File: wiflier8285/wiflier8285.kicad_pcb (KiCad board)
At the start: 2 copper layers, 37.8 x 21.5 mm, 46 parts, among them CN1 1u, CN2 1u, M0 M, M1 M, M2 M, M3 M, P1 USBMicroB-10118194-0001LF, P2 CONN_01X02, P3 I2C, P4 TXRX, P5 TXRX, P6 IVP, P7 M, P8 M, P9 SYSRESET, Q0 NFET, Q1 NFET, Q2 NFET, Q3 NFET, U1 BMP280, U2 ESP8285, U3 LSM9DS1, U4 MCP1824v3.3, U5 MCP1824v3.3, U6 MCP1824v2.5, U7 STBC08, X1 XTAL4P

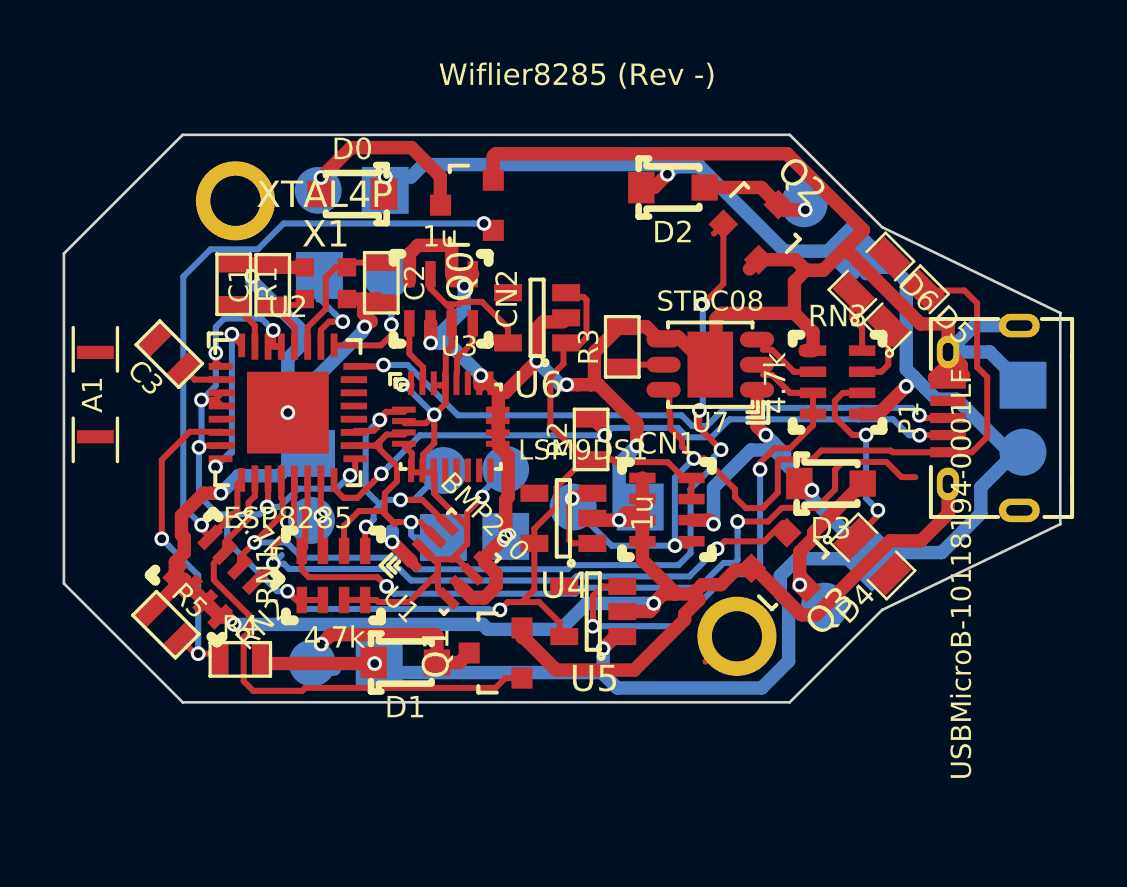
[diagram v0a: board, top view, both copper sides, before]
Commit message: Update!
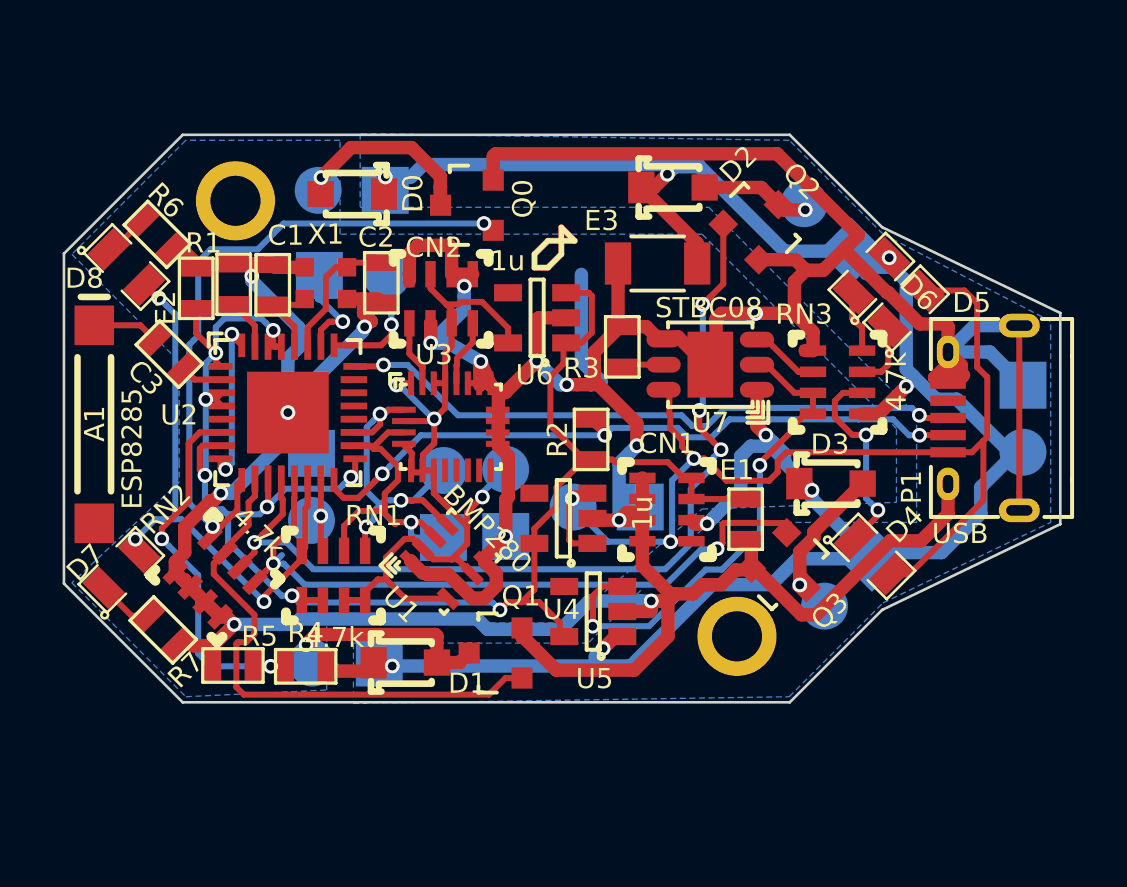
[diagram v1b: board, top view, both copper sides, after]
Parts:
- added D7: BLU, SM0805, F.Cu at (47.6, 65.7)
- added D8: BLU, SM0805, F.Cu at (47.8, 54.2)
- added E1: 10u, SM0603, F.Cu at (71.3, 63.7)
- added E2: 10u, SM0603, F.Cu at (50.5, 55.0)
- added E3: 100u, C_1206, F.Cu at (67.9, 54.1)
- added R6: 1.5k, SM0603, F.Cu at (49.0, 52.9)
- added R7: 1.5k, SM0603, F.Cu at (49.2, 67.9)
- A1: footprint ANT1206 -> RFANT8010080A3T
- P1: value USBMicroB-10118194-0001LF -> USB
- P2: value CONN_01X02 -> BATTERY
- moved R5 2.97 mm to (51.8, 69.3), turned to 0 degrees
- moved R4 2.49 mm to (54.6, 69.3)
- moved A1 1.13 mm to (46.6, 60.1)
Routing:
- net GND: track 177.6 -> 194.1 mm
- net (no net): track 4.80 -> 14.8 mm
- net G2: track 30.8 -> 21.2 mm, vias 2 -> 3
- net VI: track 37.5 -> 42.4 mm
- net +3V3: track 59.0 -> 63.9 mm
- net Net-(A1-Pad1): track 0.00 -> 2.53 mm
- net ADC: track 12.5 -> 14.7 mm
- net +2V5: track 32.3 -> 34.5 mm
- net Net-(D7-Pad1): track 0.00 -> 2.16 mm
- net Net-(D8-Pad1): track 0.00 -> 2.02 mm
- net M0: track 6.22 -> 8.09 mm
- net RX: track 3.78 -> 4.76 mm
- net PWM1: track 19.9 -> 20.8 mm
- net TX: track 2.87 -> 3.79 mm
- net EN_B: track 19.8 -> 19.1 mm
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- added copper zone on B.Cu, net BATT
- added copper zone on B.Cu, net GND
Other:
- net class Default: clearance 0.19812 -> 0.1905
- net class MP: clearance 0.2032 -> 0.1905
- rule trace_clearance: 0.19812 -> 0.1905
- board text added: "(Rev -) Wiflier8285"
- board text added: "+"
- board text added: "-"
- board text added: "0"
- board text added: "2.5"
- board text added: "5"
- board text added: "CL"
- board text added: "DA"
- board text added: "G0"
- board text added: "GND"
- board text added: "RX"
- board text added: "TX"
- board text removed: "Wiflier8285 (Rev -)"
